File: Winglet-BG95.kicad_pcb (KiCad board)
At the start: 4 copper layers, 30 x 47.6 mm, 43 parts, among them J1 2337019-1, J2 2337019-1, J3 1042240820, M1 PTH_M2.5, M2 PTH_M2.5, Q1 DMG1012UW-7, Q2 DMG1012UW-7, U1 BG95MxLA, U2 MFF2-SIM, U3 24AA01T-I/OT, U4 FXLA108BQX

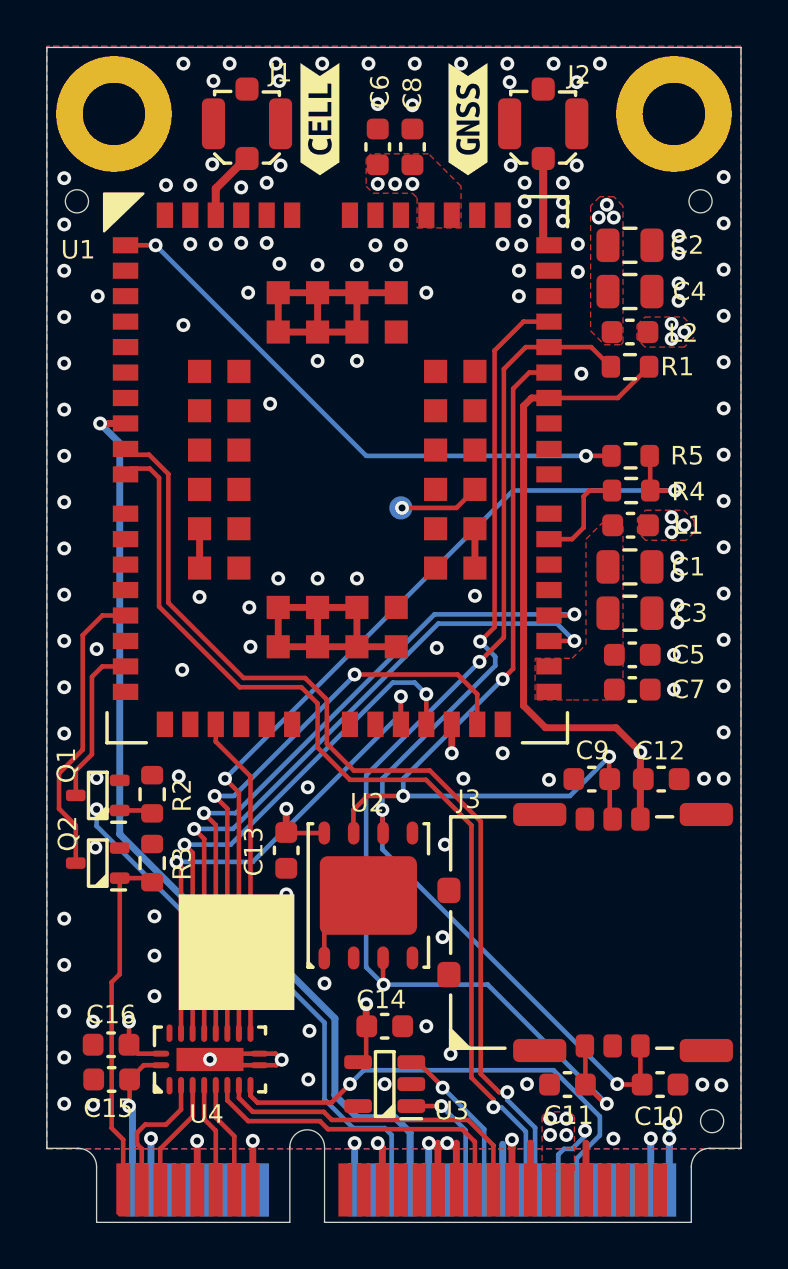
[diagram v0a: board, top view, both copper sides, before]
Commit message: Nitpicks before release
Update output scripts
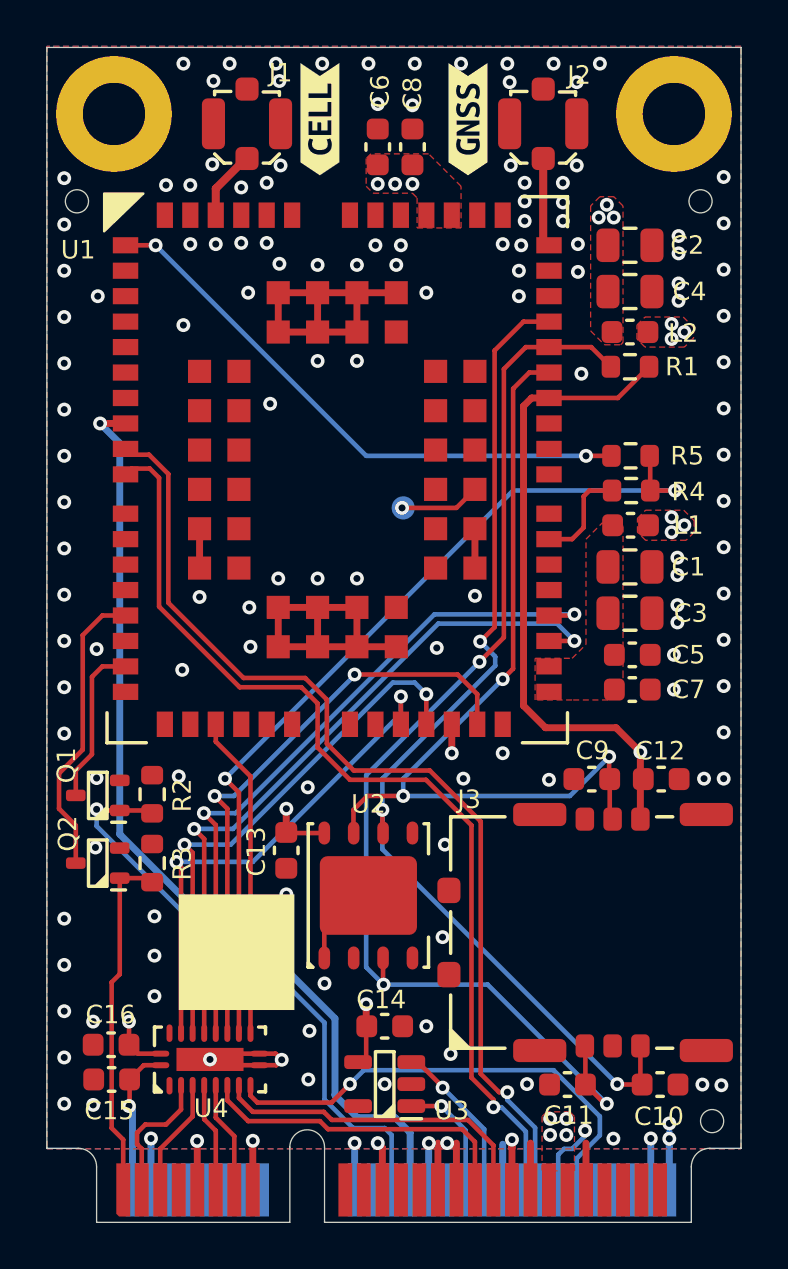
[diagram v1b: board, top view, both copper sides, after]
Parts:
- moved TP1 0.10 mm to (65.4, 69.9)
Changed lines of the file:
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@@
 			(layer "F.Mask"
 				(type "Top Solder Mask")
-				(color "Blue")
+				(color "Black")
 				(thickness 0.01)
 			)
@@
 			(layer "B.Mask"
 				(type "Bottom Solder Mask")
-				(color "Blue")
+				(color "Black")
 				(thickness 0.01)
 			)
@@
 		(at 75.2 63.8 180)
 		(property "Reference" "R1"
-			(at -2.05 0 0)
+			(at -2.25 0 0)
 			(layer "F.SilkS")
 			(effects
@@
 		(at 57.05 93.735 90)
 		(property "Reference" "U4"
-			(at -2.365 -0.15 0)
+			(at -2.115 0.05 180)
 			(layer "F.SilkS")
 			(effects
@@
 			(layer "F.Fab")
 		)
+		(fp_text user "${REFERENCE}"
+			(at 0 0 180)
+			(layer "F.Fab")
+			(effects
+				(font
+					(size 0.75 0.75)
+					(thickness 0.11)
+				)
+			)
+		)
 		(pad "1" smd oval
 			(at -0.25 -2.135)
@@
 		(at 60.345 84.7 -90)
 		(property "Reference" "C13"
-			(at 0.05 1.4 90)
+			(at 0.05 1.295 90)
 			(layer "F.SilkS")
 			(effects
@@
 		(at 52.8 94.6 180)
 		(property "Reference" "C15"
-			(at 0.145 -1.25 0)
+			(at 0.1 -1.35 0)
 			(layer "F.SilkS")
 			(effects
@@
 		(at 63.895 86.65 90)
 		(property "Reference" "U2"
-			(at 4 -0.045 180)
+			(at 3.95 0.005 180)
 			(layer "F.SilkS")
 			(effects
@@
 			(layer "F.Fab")
 		)
+		(fp_text user "${REFERENCE}"
+			(at 0 0 90)
+			(unlocked yes)
+			(layer "F.Fab")
+			(effects
+				(font
+					(size 1 1)
+					(thickness 0.15)
+				)
+			)
+		)
 		(pad "" smd roundrect
 			(at -0.8 -0.9 90)
@@
 		(at 52.775 93.1 180)
 		(property "Reference" "C16"
-			(at 0 1.3 0)
+			(at 0.025 1.3 0)
 			(layer "F.SilkS")
 			(effects
@@
 	(footprint "TP_TestPoint:TestPoint_1mm"
 		(layer "B.Cu")
-		(at 65.3 69.9 180)
+		(at 65.4 69.9 180)
 		(descr "SMD pad as test Point, diameter 1.0mm")
 		(tags "test point SMD pad")
@@
 			(effects
 				(font
-					(size 0.8 0.8)
+					(size 1 1)
 					(thickness 0.15)
 				)
@@
 			(end 0 -0.7)
 			(stroke
-				(width 0.12)
+				(width 0.15)
 				(type solid)
 			)
@@
 			(layer "B.CrtYd")
 		)
+		(fp_circle
+			(center 0 0)
+			(end 0.7 0)
+			(stroke
+				(width 0.1)
+				(type default)
+			)
+			(fill no)
+			(layer "B.Fab")
+		)
 		(fp_text user "${REFERENCE}"
